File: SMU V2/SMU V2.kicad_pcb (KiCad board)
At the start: 4 copper layers, 94.8 x 90.7 mm, 86 parts, among them J1101 SMA, J1201 SMA, J401 Connector, J402 Connector, Q1201 SI2301CDS-T1-GE3, U1001 TPS5430DDAR, U1002 ETQ-P3M150KVN, U1301 Display, U1401 AMS1117-3.3, U601 LSM6DSOTR, U701 TPS7A2033PDBVR, U801 TPS7A2033PDBVR, U901 TPS7A2033PDBVR

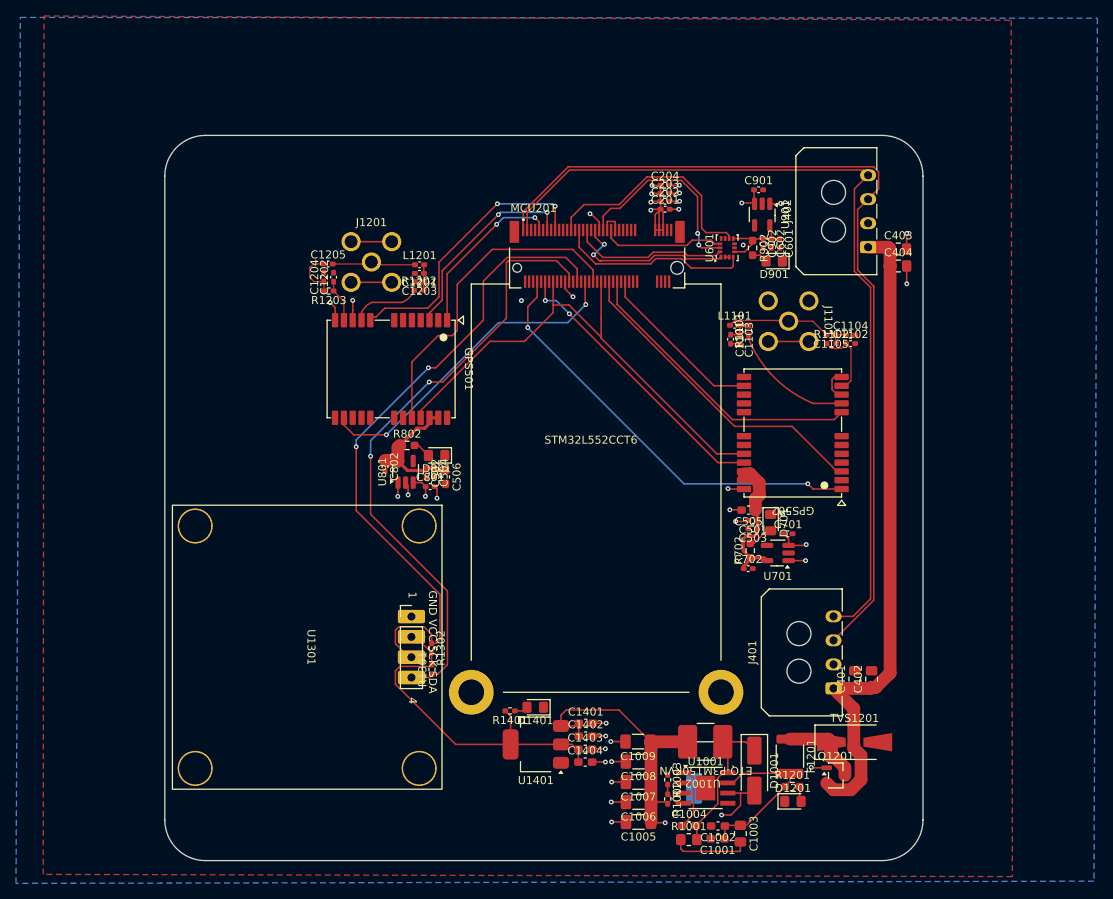
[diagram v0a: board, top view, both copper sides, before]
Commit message: test
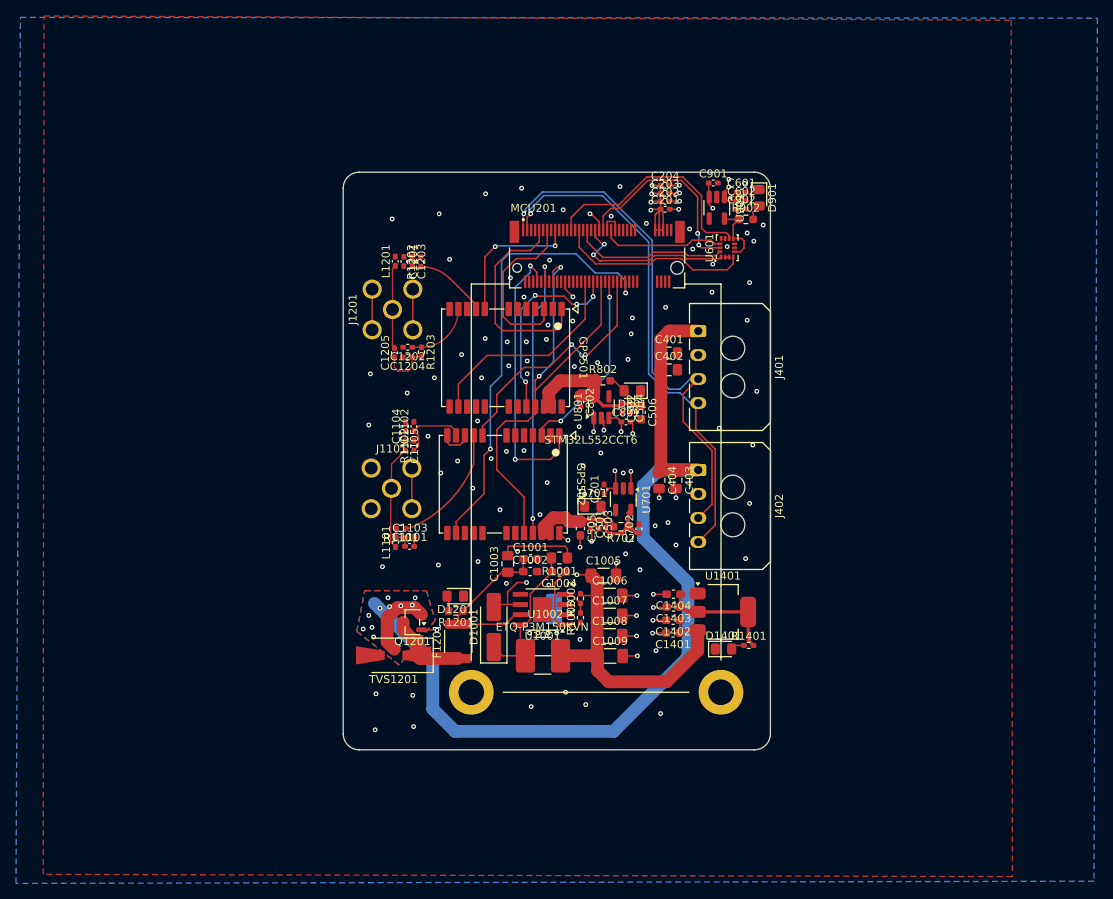
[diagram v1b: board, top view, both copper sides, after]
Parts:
- removed R1301, R1302: 4.7k, Resistor_SMD:R_0402_1005Metric_Pad0.72x0.64mm_HandSolder
- removed U1301: Display, bfr_utilities:1.3 OLED Display
- moved TVS1201 58.6 mm to (130.8, 115.6), turned to 180 degrees
- moved C1104 56.8 mm to (132.3, 87.0), turned to 90 degrees
- moved Q1201 56.3 mm to (133.1, 111.4), turned to 180 degrees
- moved C1102 55.6 mm to (133.3, 87.0), turned to 90 degrees
- moved C1105 55.0 mm to (132.2, 89.4), turned to -90 degrees
- moved J1101 53.9 mm to (130.5, 94.7), turned to 0 degrees
- moved R1102 53.7 mm to (133.3, 89.4), turned to 90 degrees
- moved L1101 50.3 mm to (131.0, 101.5), turned to 90 degrees
- moved R1101 50.0 mm to (131.7, 99.7), turned to 180 degrees
- moved D1201 49.4 mm to (138.5, 108.2), turned to 180 degrees
- moved C1103 48.1 mm to (132.8, 100.8), turned to 0 degrees
- moved J401 47.8 mm to (168.9, 75.0), turned to -90 degrees
- moved C1101 47.8 mm to (132.8, 102.0), turned to 0 degrees
- moved R1201 47.4 mm to (138.6, 110.0), turned to 180 degrees
- moved C401 46.9 mm to (165.2, 77.8), turned to 0 degrees
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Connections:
- net /GPS1.UART_TX renamed /GPS2.UART_RX
- MCU201 pad 24: /DISP_I2C_SDA -> /Microcontroller/DISP_I2C_SDA
- MCU201 pad 28: /DISP_I2C_SCL -> /Microcontroller/DISP_I2C_SCL
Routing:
- net /DISP_I2C_SCL: track 84.0 -> 0.00 mm, vias 2 -> 0
- net /DISP_I2C_SDA: track 77.0 -> 0.00 mm, vias 2 -> 0
- net /CAN+: track 111.9 -> 66.0 mm, vias 0 -> 1
- net /CAN-: track 107.3 -> 64.4 mm, vias 0 -> 1
- net /Main IO/VBATT+: track 81.7 -> 120.8 mm, vias 0 -> 10
- net /GPS1.ANT_ON: track 21.4 -> 56.6 mm, vias 0 -> 2
- net +3V3: track 46.6 -> 14.8 mm
- net /GPS1.WKUP: track 53.8 -> 35.2 mm
- net /GPS2.RST: track 34.8 -> 17.9 mm
- net /GPS1.1PPS: track 40.3 -> 23.6 mm, vias 0 -> 2
- net /GPS2.UART_TX: track 41.4 -> 25.0 mm, vias 0 -> 4
- net /GPS2.ANT_ON: track 41.4 -> 26.7 mm, vias 2 -> 0
- net GND: track 78.5 -> 70.9 mm, vias 29 -> 116
- net /GPS1.RST: track 37.2 -> 31.3 mm, vias 0 -> 2
- net /GPS2.UART_RX: track 65.0 -> 59.1 mm, vias 0 -> 2
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- added copper zone on B.Cu, net /Main IO/VBATT+
- added copper zone on F.Cu, net /Main IO/VBATT+
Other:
- board size 94.8 x 90.7 mm -> 53.4 x 72.2 mm
